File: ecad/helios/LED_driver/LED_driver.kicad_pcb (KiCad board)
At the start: 2 copper layers, 67.2 x 100 mm, 101 parts, among them J1 Conn_02x04_Top_Bottom, J2 Conn_02x03_Top_Bottom, J3 Conn_02x04_Top_Bottom, J4 Conn_02x03_Odd_Even, Q1 IRF9Z34NPbF, Q2 PMV48XP,215, SW1 SW_Push, U1 UA9637, U2 TPS92512, U3 TPS92512, U4 TPS92512, U5 TPS1H100AQ, U6 LM2936-5.0, U7 ATTINY24-20SSU, Y1 10 MHz

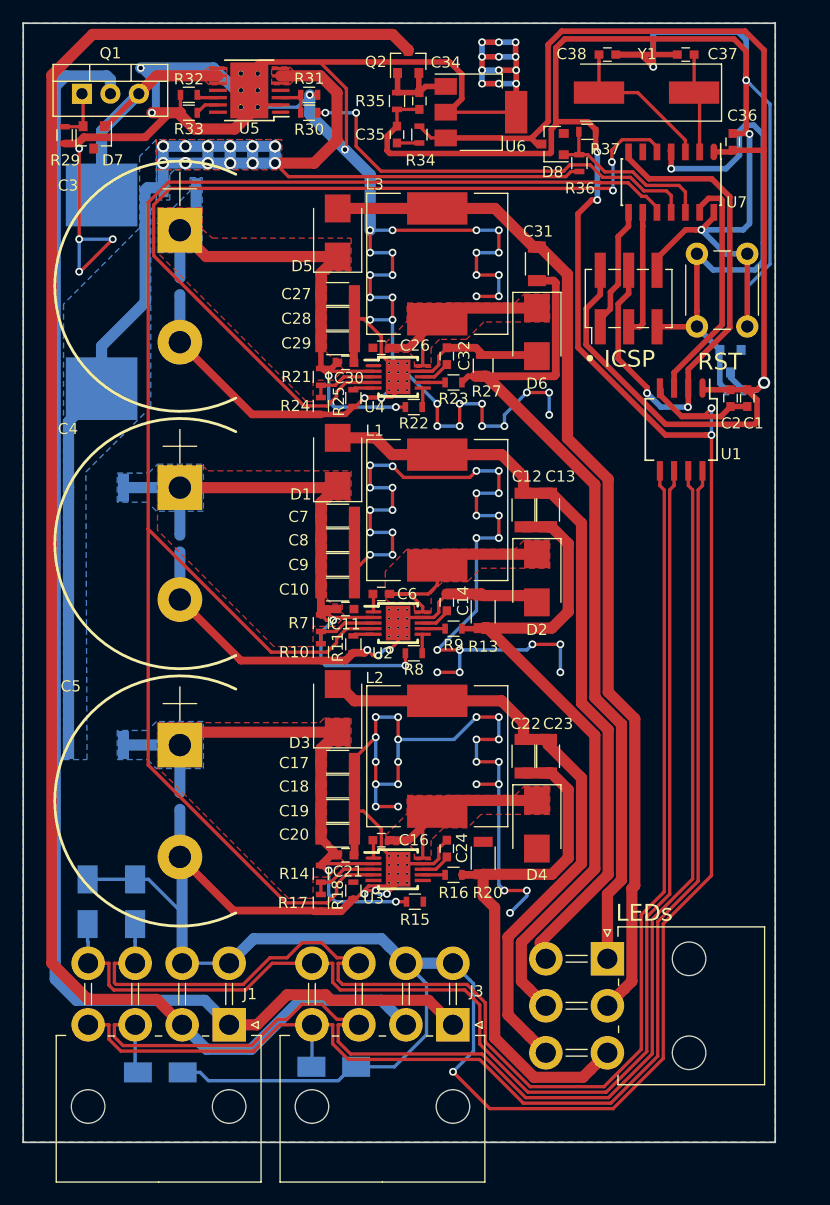
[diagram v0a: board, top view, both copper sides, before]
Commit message: Improves the layout
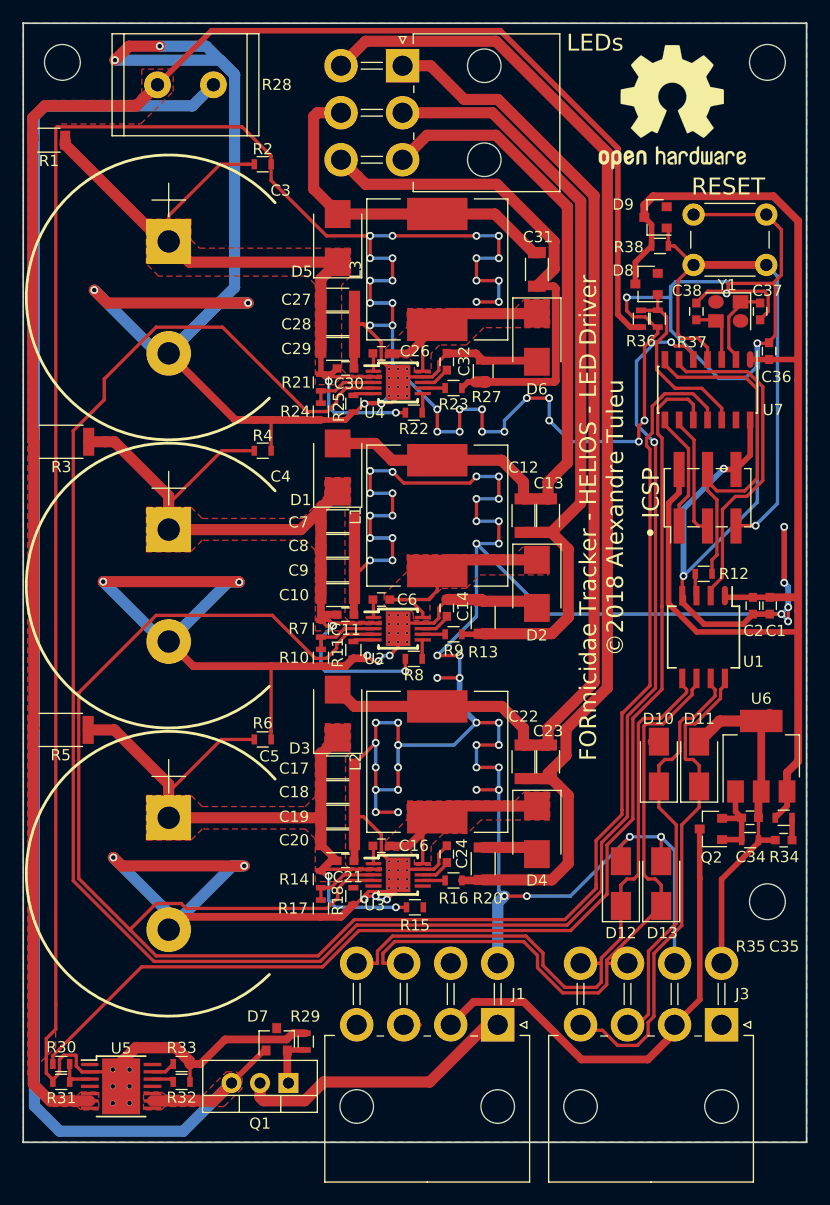
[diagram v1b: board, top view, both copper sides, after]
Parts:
- added R12: 100, Resistors_SMD:R_0603, F.Cu at (110.8, 92.7)
- added REF**: MountingHole_3.2mm_M3_DIN965, Mounting_Holes:MountingHole_3.2mm_M3_DIN965, F.Cu at (53.5, 47.0)
- added REF**: MountingHole_3.2mm_M3_DIN965, Mounting_Holes:MountingHole_3.2mm_M3_DIN965, F.Cu at (116.5, 122.0)
- added REF**: MountingHole_3.2mm_M3_DIN965, Mounting_Holes:MountingHole_3.2mm_M3_DIN965, F.Cu at (116.5, 47.0)
- added REF***: OSHW-Logo2_14.6x12mm_SilkScreen, Symbols:OSHW-Logo2_14.6x12mm_SilkScreen, F.Cu at (108.0, 51.0)
- C3, C4, C5: footprint FORT:CP_Radial_D22.0mm_P10.00mm_SnapIn -> FORT:CP_Radial_D25.0mm_P10.00mm_H32mm_SnapIn
- D10, D11, D12, D13, D9, R1, R2, R3, R38, R4, R5, R6: moved to F.Cu
- J1, J3: footprint Connectors_Molex:Molex_MiniFit-JR-5569-08A2_2x04x4.20mm_Angled -> FORT:Molex_MiniFit-JR-5569-08A2_2x04x4.20mm_Angled
- J2: footprint Connectors_Molex:Molex_MiniFit-JR-5569-06A2_2x03x4.20mm_Angled -> FORT:Molex_MiniFit-JR-5569-06A2_2x03x4.20mm_Angled
- L1, L2, L3: footprint Inductors_SMD:L_Wuerth_WE-PD-Typ-LS -> FORT:7447709101
- R28: value 47, 4W -> 47, 5W; footprint FORT:R_S-5 -> Resistors_THT:R_Radial_Power_L13.0mm_W9.0mm_P5.00mm; moved to F.Cu
- Y1: footprint Crystals:Crystal_SMD_HC49-SD -> Crystals:Crystal_SMD_TXC_7M-4pin_3.2x2.5mm
- moved R31 90.9 mm to (53.4, 138.1), turned to 180 degrees
- moved Q1 90.3 mm to (73.7, 138.2), turned to 180 degrees
- moved U5 89.7 mm to (58.8, 138.5), turned to 0 degrees
- moved R32 88.2 mm to (64.2, 138.1), turned to 0 degrees
- moved R30 87.8 mm to (53.4, 136.5), turned to 180 degrees
- moved R33 85.0 mm to (64.2, 136.5), turned to 0 degrees
- moved R29 83.8 mm to (75.2, 134.5), turned to 90 degrees
- moved D7 82.2 mm to (72.7, 134.3), turned to 90 degrees
- moved J2 81.9 mm to (83.9, 47.3)
- moved Q2 73.7 mm to (111.5, 115.5), turned to 180 degrees
- moved R35 73.2 mm to (115.0, 116.5), turned to 0 degrees
- moved C35 71.9 mm to (118.0, 116.5), turned to 180 degrees
- moved C34 70.5 mm to (115.0, 114.5), turned to 0 degrees
- moved R34 69.2 mm to (118.0, 114.5), turned to 0 degrees
- moved U6 62.8 mm to (116.0, 109.0), turned to 90 degrees
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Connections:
- D10 pad 1: /DATA_- -> /IR_ON_-
- D11 pad 1: /DATA_+ -> /IR_ON_+
- D12 pad 1: /IR_ON_- -> /DATA_-
- D13 pad 1: /IR_ON_+ -> /DATA_+
- J1 pad 3: /DATA_- -> /IR_ON_-
- J1 pad 4: /DATA_+ -> /IR_ON_+
- J1 pad 7: /IR_ON_- -> /DATA_+
- J1 pad 8: /IR_ON_+ -> /DATA_-
- J2 pad 1: /VIS- -> /IRB+
- J2 pad 2: /VIS+ -> /IRA-
- J2 pad 3: /IRB- -> /IRA+
- J2 pad 4: /IRA+ -> /IRB-
- J2 pad 5: /IRA- -> /VIS+
- J2 pad 6: /IRB+ -> /VIS-
- J3 pad 3: /DATA_- -> /IR_ON_-
- J3 pad 4: /DATA_+ -> /IR_ON_+
- J3 pad 7: /IR_ON_- -> /DATA_+
- J3 pad 8: /IR_ON_+ -> /DATA_-
- J4 pad 4: /Controller/DATA_IN -> /Controller/ICSP_MOSI
- U1 pad 2: /Controller/DATA_IN -> /Controller/FLASH_IN
- U1 pad 3: /Controller/FLASH_IN -> /Controller/DATA_IN
- U1 pad 5: /IR_ON_- -> /DATA_-
- U1 pad 6: /IR_ON_+ -> /DATA_+
- U1 pad 7: /DATA_- -> /IR_ON_-
- U1 pad 8: /DATA_+ -> /IR_ON_+
- U7 pad 10: /Controller/IR_ON -> /Power_Management.sch/EN36
- U7 pad 11: /Power_Management.sch/EN36 -> /Controller/IR_ON
- U7 pad 13: /Controller/FLASH_IN -> Net-(U7-Pad13)
- U7 pad 6: Net-(U7-Pad6) -> /Controller/FLASH_IN
- U7 pad 7: /Controller/DATA_IN -> /Controller/ICSP_MOSI
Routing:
- net /Power_Management.sch/V36_PROTECTED: track 22.4 -> 137.9 mm
- net /VS6: track 150.9 -> 43.1 mm
- net /Buck_Current_regulator_1A_1/PDIM: track 81.4 -> 185.7 mm
- net /VS36: track 125.9 -> 25.5 mm
- net /IR_ON_-: track 123.2 -> 41.3 mm
- net /IR_ON_+: track 119.3 -> 47.0 mm
- net /Power_Management.sch/EN36: track 38.6 -> 107.6 mm, vias 2 -> 0
- net /DATA_-: track 123.5 -> 60.4 mm
- net /VIS+: track 91.8 -> 31.7 mm
- net /IRB-: track 48.3 -> 107.8 mm
- net /DATA_+: track 118.8 -> 61.1 mm
- net /Controller/DATA_IN: track 48.0 -> 2.60 mm, vias 2 -> 0
- net +36V: track 127.9 -> 169.7 mm, vias 12 -> 0
- net /IRB+: track 55.1 -> 94.4 mm
- net /Controller/ICSP_MOSI: track 0.00 -> 34.3 mm
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- removed copper zone on B.Cu, net +36V
- removed copper zone on B.Cu, net /Buck_Current_regulator_1.5A_1/VIN
- removed copper zone on B.Cu, net /Buck_Current_regulator_1.5A_2/VIN
- removed copper zone on B.Cu, net /Buck_Current_regulator_1A_1/VIN
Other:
- board size 67.2 x 100 mm -> 70 x 100 mm
- board text added: "FORmicidae Tracker - HELIOS - LED Driver ©2018 Alexandre Tuleu"
- board text added: "RESET"
- board text removed: "RST"
